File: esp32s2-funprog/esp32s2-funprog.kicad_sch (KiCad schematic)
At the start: 97 parts, among them J1 OPGM, J2 PGM, J3 USB_C_Receptacle_USB2.0, J4 MOUNT, J5 MOUNT, Q1 SE4625-PandN, Q2 SE4625-PandN, Q3 DWL336C, Q4 2N7002, Q6 2N7002KDW, Q7 MOT2302, SW1 TS-1187A-B-A-B, U1 ESP32-S2, U10 LM321, U11 ZDT6790TA, U12 COS4514, U14 AT8837, U15 AT8837, U16 AT8837, U2 XC6206P332, U3 MT3608, U4 XC6206P332, U5 COSNE5532, U6 XC6206P332, U8 HP3000, U9 AT8837, Y1 40MHz

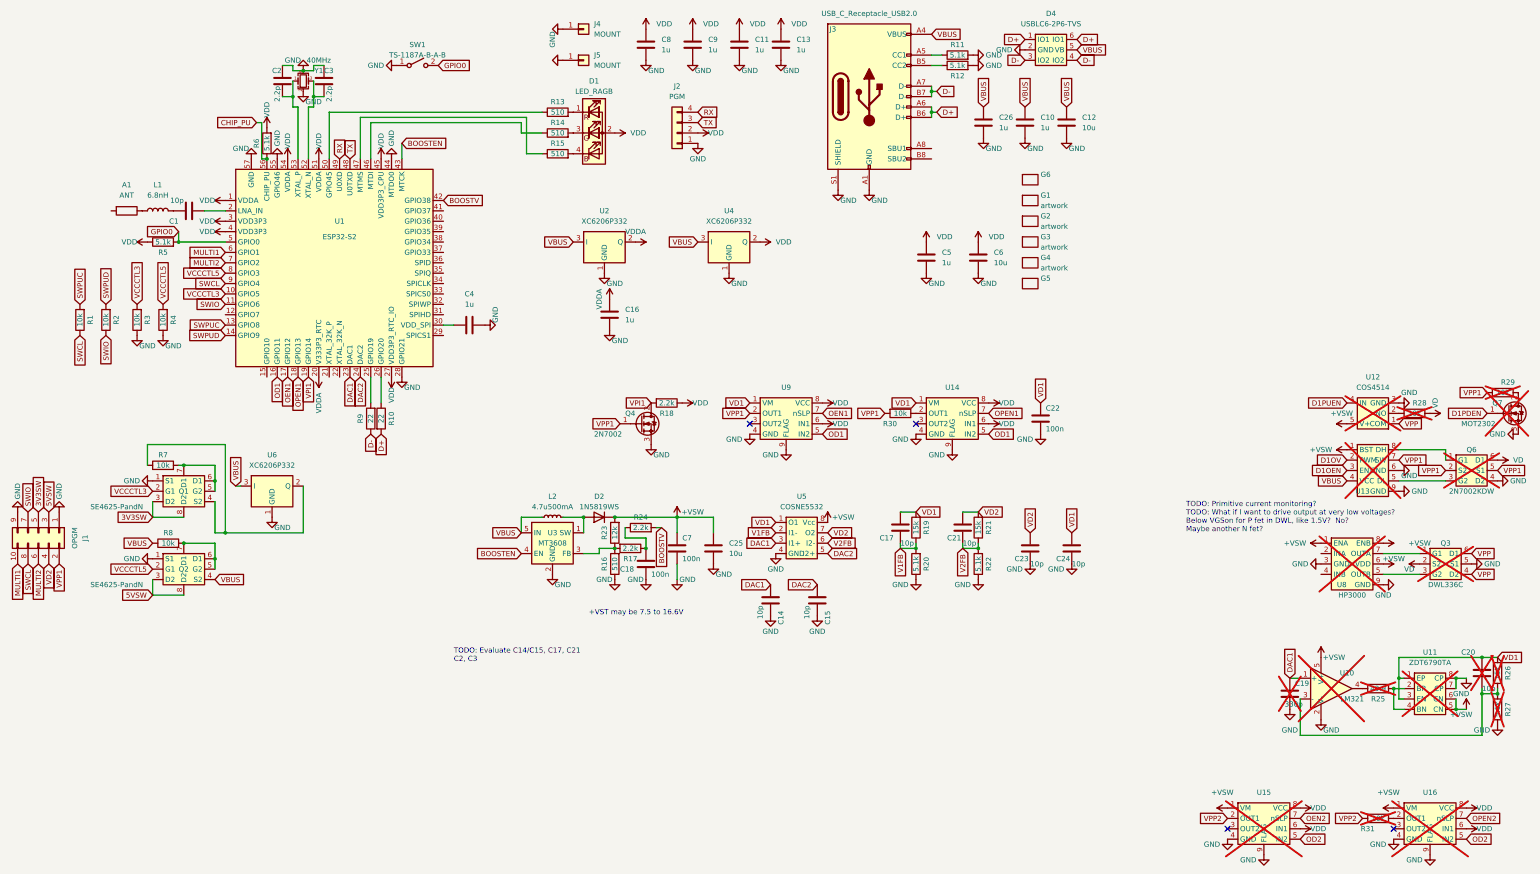
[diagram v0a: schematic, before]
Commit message: Bump - back to legacy
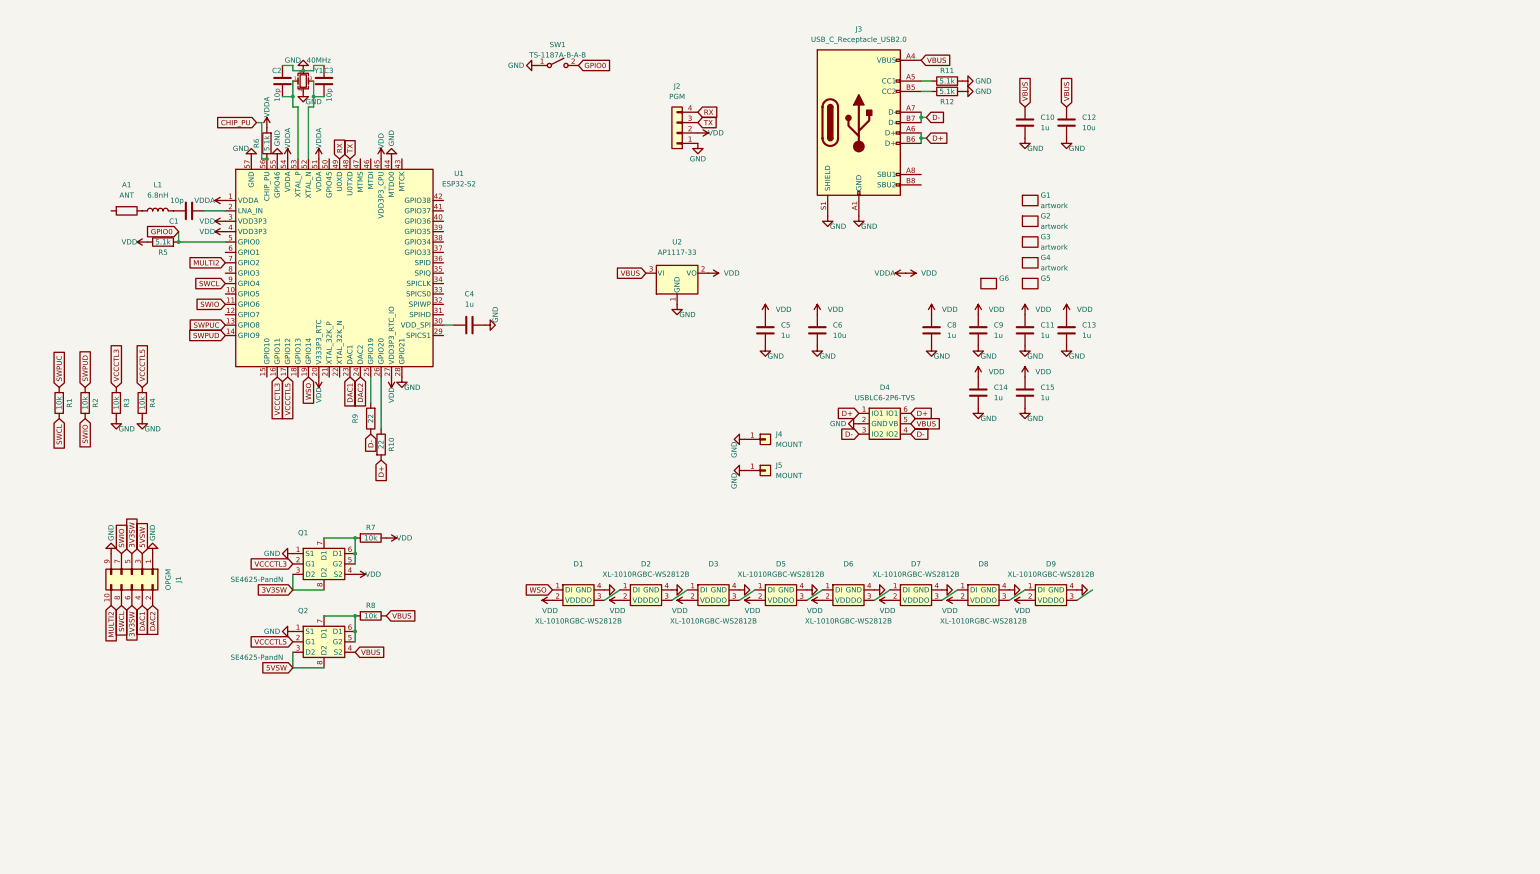
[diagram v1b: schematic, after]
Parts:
- removed C16, C26: 1u, Capacitor_SMD:C_0402_1005Metric, symbol Device:C
- removed C17, C20, C21, C23, C24: 10p, Capacitor_SMD:C_0402_1005Metric, symbol Device:C
- removed C18, C22, C7: 100n, Capacitor_SMD:C_0402_1005Metric, symbol Device:C
- removed C19: 330p, Capacitor_SMD:C_0402_1005Metric, symbol Device:C
- removed C25: 10u, Capacitor_SMD:C_0603_1608Metric, symbol Device:C
- removed D1: LED_RAGB, LED_SMD:LED_WS2812B-2020_PLCC4_2.0x2.0mm, symbol Device:LED_RAGB
- removed D2: 1N5819WS, Diode_SMD:D_SOD-323, symbol Device:D
- removed L2: 4.7u500mA, Inductor_SMD:L_0805_2012Metric, symbol Device:L_Small
- removed Q3: DWL336C, Package_TO_SOT_SMD:SOT-23-6, symbol cnhardware:DWL336C-P-AND-N
- removed Q4: 2N7002, Package_TO_SOT_SMD:SOT-23, symbol Device:Q_NMOS_GDS
- removed Q6: 2N7002KDW, Package_TO_SOT_SMD:SOT-363_SC-70-6, symbol cnhardware:DWL336C-P-AND-N
- removed Q7: MOT2302, Package_TO_SOT_SMD:SOT-23, symbol Device:Q_NMOS_GDS
- removed R13, R14, R15, R16: 510, Resistor_SMD:R_0402_1005Metric, symbol Device:R
- removed R17, R18, R24: 2.2k, Resistor_SMD:R_0402_1005Metric, symbol Device:R
- removed R19, R21, R26: 15k, Resistor_SMD:R_0402_1005Metric, symbol Device:R
- removed R20, R22, R27: 5.1k, Resistor_SMD:R_0402_1005Metric, symbol Device:R
- removed R23: 12k, Resistor_SMD:R_0402_1005Metric, symbol Device:R
- removed R25: 49.9, Resistor_SMD:R_0402_1005Metric, symbol Device:R
- removed R28, R29, R30, R31: 10k, Resistor_SMD:R_0402_1005Metric, symbol Device:R
- removed U10: LM321, Package_TO_SOT_SMD:SOT-23-5, symbol Amplifier_Operational:LM321
- removed U11: ZDT6790TA, Package_TO_SOT_SMD:SOT-223-8, symbol cnhardware:ZDT6790-COMPLEMENTARY-BJT
- removed U12: COS4514, Package_TO_SOT_SMD:SOT-23-5, symbol cnhardware:COS4514-MUX-SPST
- removed U13: ~, Package_DFN_QFN:DFN-8-1EP_3x3mm_P0.5mm_EP1.65x2.38mm, symbol cnhardware:NCP81155-GATE-DRIVER
- removed U14, U15, U16, U9: AT8837, Package_DFN_QFN:DFN-8-1EP_2x2mm_P0.45mm_EP0.64x1.38mm, symbol cnhardware:BDR6122TC-MOTOR-DRIVER
- removed U2, U4, U6: XC6206P332, Package_TO_SOT_SMD:SOT-23, symbol Regulator_Linear:IFX27001TFV26
- removed U3: MT3608, Package_TO_SOT_SMD:SOT-23-6, symbol Regulator_Switching:MT3608
- removed U5: COSNE5532, Package_SO:MSOP-8_3x3mm_P0.65mm, symbol cnhardware:LM2903-SOIC8
- removed U8: HP3000, Package_DFN_QFN:DFN-8-1EP_2x2mm_P0.5mm_EP0.6x1.2mm, symbol cnhardware:HP3000-AD000-HD08R-DUAL-LOW-DRIVER
- added D1, D2, D3, D5, D6, D7, D8, D9: XL-1010RGBC-WS2812B, cnhardware:XL-1010RGBC-WS812B, symbol cnhardware:SK6805-EC15
- added U2: AP1117-33, Package_TO_SOT_SMD:SOT-223-3_TabPin2, symbol Regulator_Linear:AP1117-33
- C14, C15: value 10p -> 1u; LCSC C106199 -> C106254
- C2, C3: value 2.2p -> 10p; LCSC C1559 -> C106199
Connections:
- net OD1 is gone; now on net VCCCTL3: U1.16 (GPIO11)
- net OEN1 is gone; now on net VCCCTL5: U1.17 (GPIO12)
- net VD2 is gone; now on net DAC1: J1.4 (Pin_4)
- net VDDA is gone; now on net VDD: U1.20 (V333P3_RTC)
- net VPP1 is gone; now on net DAC2: J1.2 (Pin_2)
- net 3V3SW: now also J1.6 (Pin_6)
- net DAC1: no longer C14.2
- net DAC2: no longer C15.2
- net GND: now also C14.2, C15.2, D1.4 (GND), D2.4 (GND), D3.4 (GND), D5.4 (GND), D6.4 (GND), D7.4 (GND), D8.4 (GND), D9.4 (GND), U2.1 (GND); no longer C14.1, C15.1
- net MULTI2: now also J1.10 (Pin_10); no longer J1.6 (Pin_6)
- net VBUS: now also U2.3 (VI)
- net VCCCTL3: no longer U1.10 (GPIO5)
- net VCCCTL5: no longer U1.8 (GPIO3)
- net VDD: now also C14.1, C15.1, Q1.4 (S2), R7.1, D1.2 (VDD), D2.2 (VDD), D3.2 (VDD), D5.2 (VDD), D6.2 (VDD), D7.2 (VDD), D8.2 (VDD), D9.2 (VDD), U2.2 (VO)
- net BOOSTEN: no longer names the net of U1.43 (MTCK)
- net BOOSTV: no longer names the net of U1.42 (GPIO38)
- net MULTI1: no longer names the net of U1.6 (GPIO1)
- net MULTI1: no longer J1.10 (Pin_10)
- net OPEN1: no longer names the net of U1.18 (GPIO13)
- net VPI1 renamed WSO
- net WSO: now also D1.1 (DI)
- new net: D5.3 (DO), D6.1 (DI)
- new net: D6.3 (DO), D7.1 (DI)
- new net: D3.3 (DO), D5.1 (DI)
- new net: D7.3 (DO), D8.1 (DI)
- new net: D1.3 (DO), D2.1 (DI)
- new net: D2.3 (DO), D3.1 (DI)
- new net: D8.3 (DO), D9.1 (DI)
- no-connect marks 4 -> 0
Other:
- note removed: "+VST may be 7.5 to 16.6V"
- note removed: "TODO: Evaluate C14/C15, C17, C21 C2, C3"
- note removed: "TODO: Primitive current monitoring? TODO: What if I want to drive output at very low voltages? Below VGSon for P fet in DWL, like 1.5V? No? Maybe another N fet?"
- moved on the sheet: C11, C13, C5, C6, C8, C9, D4, G6, J1, J3, J4, J5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
